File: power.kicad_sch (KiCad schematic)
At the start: 33 parts, among them U17 TPS62933, U6 TLV62569DBV, U8 INA190A2IDCKR, U9 TPS2121RUXR

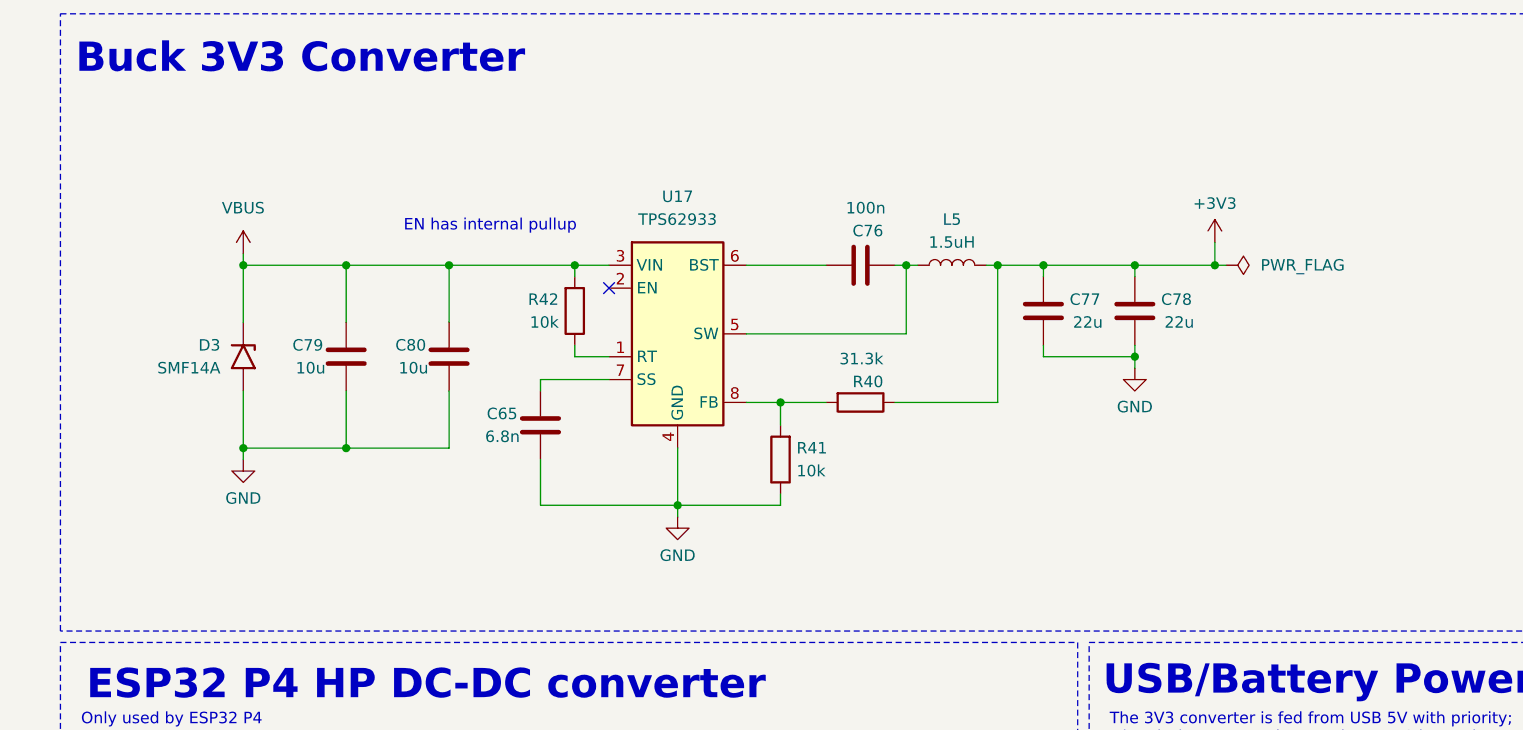
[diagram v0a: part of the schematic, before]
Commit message: Route PMW3901B
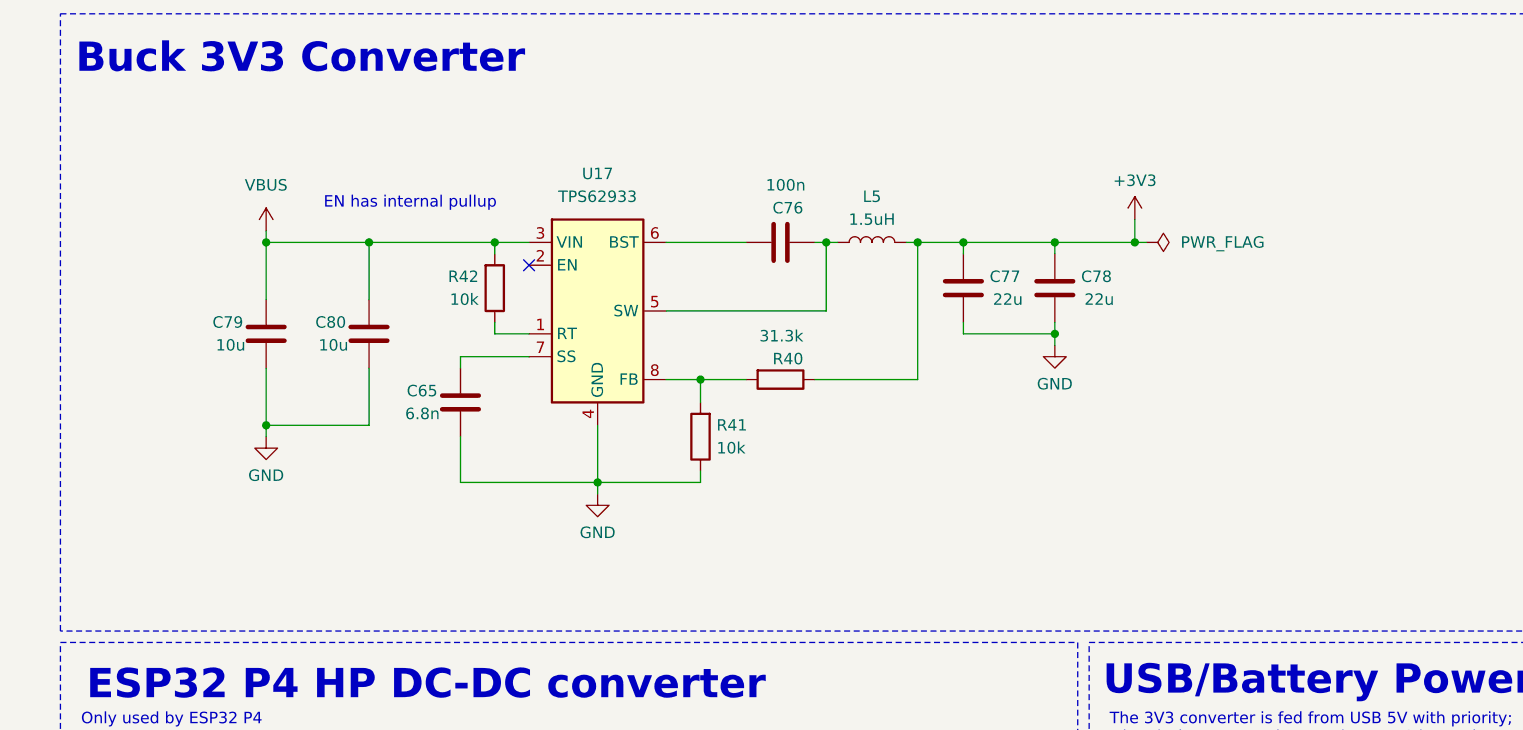
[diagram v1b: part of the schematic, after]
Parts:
- removed D3: SMF14A, Diode_SMD:D_SMF, symbol Diode:SMF14A
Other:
- moved on the sheet: C65, C76, C77, C78, C79, C80, L5, R40, R41, R42, U17
